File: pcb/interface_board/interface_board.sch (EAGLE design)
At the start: 100 parts, among them IC1 V7805-1000, IC6 LAN9512-JZX, K1 61400416021, Q6 CTS_32X25_SMD, U1 SFW15R-1STE1LF, U2 SFW15R-1STE1LF, U3 DMG1012T, U5 PAM2306DYPAA

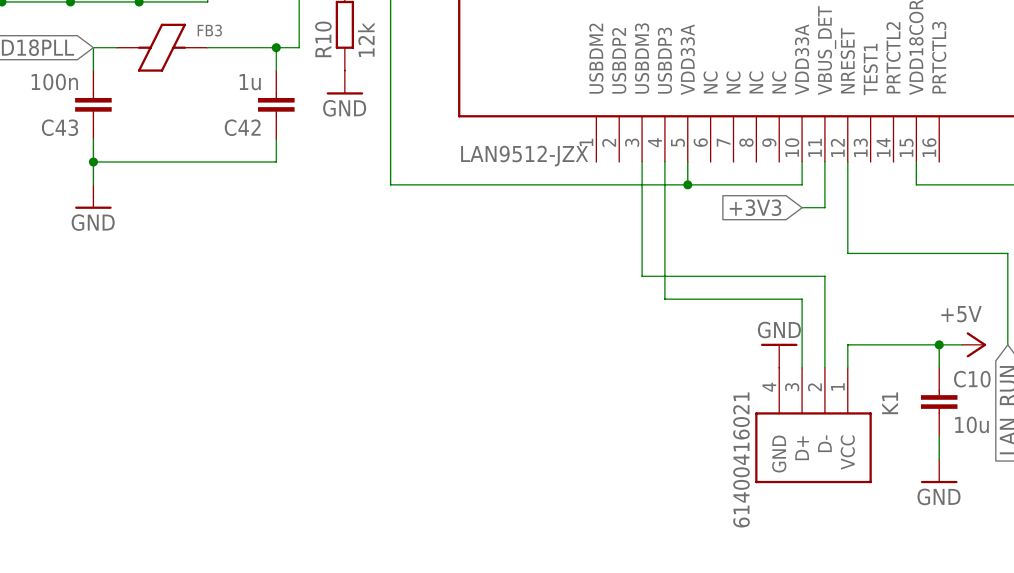
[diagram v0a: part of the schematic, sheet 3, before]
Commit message: interface_board
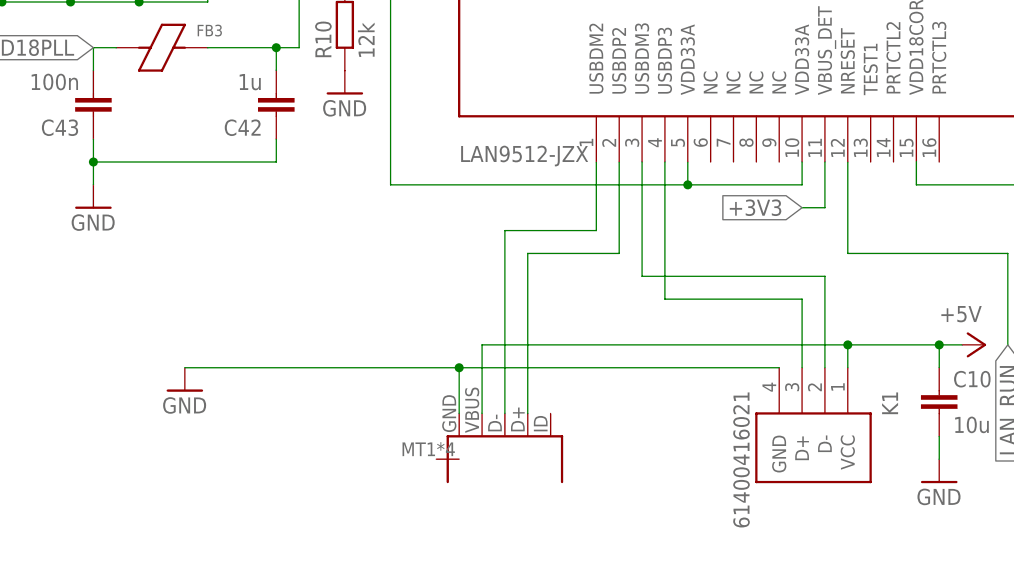
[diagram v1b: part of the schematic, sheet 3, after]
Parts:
- added JP5: USB-IDMICRO, openblw:USB-IDMICRO
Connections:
- new net N$47: IC6.USBDM2, JP5.D-
- new net N$48: IC6.USBDP2, JP5.D+
- net +5V: now also JP5.VBUS
- net GND: now also JP5.GND
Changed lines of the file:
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@@
 <part name="Q6" library="raspi" deviceset="CTS_32X25_SMD" device=""/>
 <part name="GND53" library="supply1" deviceset="GND" device=""/>
+<part name="JP5" library="openblw" deviceset="USB-ID" device="MICRO"/>
 </parts>
 <sheets>
@@
 <instance part="C10" gate="G$1" x="294.64" y="60.96"/>
 <instance part="GND9" gate="1" x="294.64" y="50.8"/>
-<instance part="GND12" gate="1" x="276.86" y="66.04" rot="R180"/>
+<instance part="GND12" gate="1" x="210.82" y="60.96"/>
 <instance part="P+8" gate="1" x="299.72" y="66.04" rot="R270"/>
 <instance part="GND32" gate="1" x="317.5" y="91.44"/>
@@
 <instance part="Q6" gate="G$2" x="175.26" y="68.58" rot="R90"/>
 <instance part="GND53" gate="1" x="157.48" y="73.66" rot="R270"/>
+<instance part="JP5" gate="G$1" x="241.3" y="55.88" rot="R270"/>
 </instances>
 <busses>
@@
 <pinref part="GND12" gate="1" pin="GND"/>
 <pinref part="K1" gate="G$1" pin="GND"/>
+<wire x1="210.82" y1="63.5" x2="241.3" y2="63.5" width="0.1524" layer="91"/>
+<pinref part="JP5" gate="G$1" pin="GND"/>
+<wire x1="241.3" y1="63.5" x2="276.86" y2="63.5" width="0.1524" layer="91"/>
+<wire x1="241.3" y1="58.42" x2="241.3" y2="63.5" width="0.1524" layer="91"/>
+<junction x="241.3" y="63.5"/>
 </segment>
 <segment>
@@
 <junction x="294.64" y="66.04"/>
 <pinref part="K1" gate="G$1" pin="VCC"/>
+<pinref part="JP5" gate="G$1" pin="VBUS"/>
+<wire x1="243.84" y1="58.42" x2="243.84" y2="66.04" width="0.1524" layer="91"/>
+<wire x1="243.84" y1="66.04" x2="284.48" y2="66.04" width="0.1524" layer="91"/>
+<junction x="284.48" y="66.04"/>
 </segment>
 </net>
@@
 </segment>
 </net>
+<net name="N$47" class="0">
+<segment>
+<pinref part="JP5" gate="G$1" pin="D-"/>
+<wire x1="246.38" y1="58.42" x2="246.38" y2="78.74" width="0.1524" layer="91"/>
+<pinref part="IC6" gate="G$1" pin="USBDM2"/>
+<wire x1="246.38" y1="78.74" x2="256.54" y2="78.74" width="0.1524" layer="91"/>
+<wire x1="256.54" y1="78.74" x2="256.54" y2="86.36" width="0.1524" layer="91"/>
+</segment>
+</net>
+<net name="N$48" class="0">
+<segment>
+<pinref part="JP5" gate="G$1" pin="D+"/>
+<wire x1="248.92" y1="58.42" x2="248.92" y2="76.2" width="0.1524" layer="91"/>
+<pinref part="IC6" gate="G$1" pin="USBDP2"/>
+<wire x1="248.92" y1="76.2" x2="259.08" y2="76.2" width="0.1524" layer="91"/>
+<wire x1="259.08" y1="76.2" x2="259.08" y2="86.36" width="0.1524" layer="91"/>
+</segment>
+</net>
